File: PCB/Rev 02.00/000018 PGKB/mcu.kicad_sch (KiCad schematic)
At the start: 30 parts, among them U5 RP2040, Y1 12 MHz

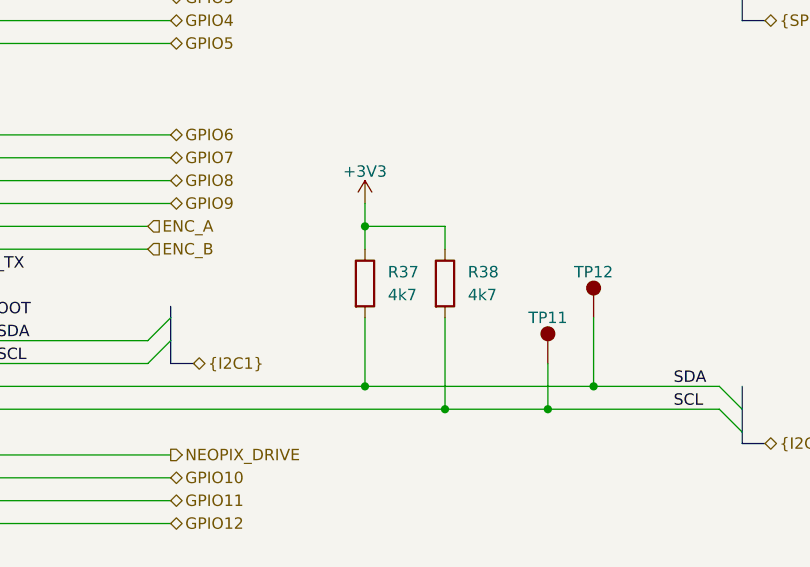
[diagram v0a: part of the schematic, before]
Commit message: step
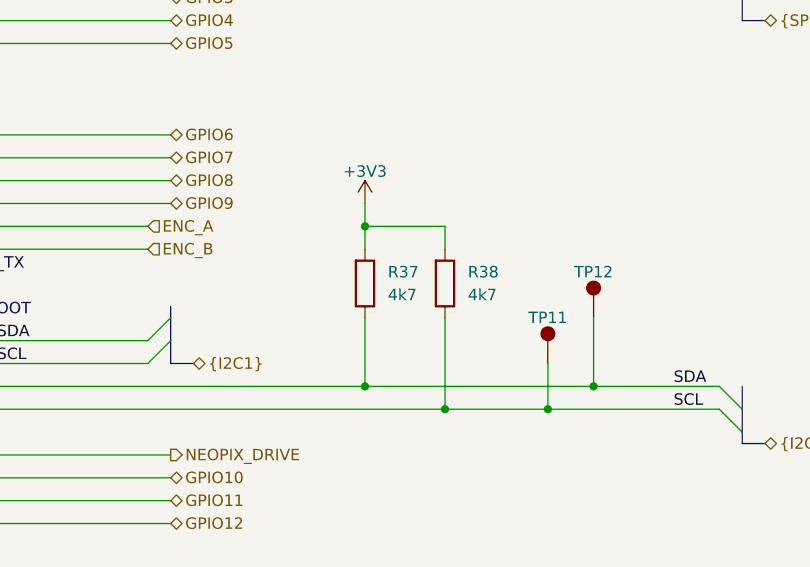
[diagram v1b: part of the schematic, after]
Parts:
- R37, R38: value R_0805_4700_5% -> 4k7; footprint KD_Resistor:RESC2012X50N -> KD_Resistor:RESC1005X40N; symbol KD_Resistor:R_0805_4700_5% -> KD_Resistor:R_0402_4700_1%; MFG_PartNo RMCF0805JT4K70 -> CR0402-FX-4701GLF; Manufacturer Stackpole Electronics Inc -> Bourns Inc.; Supplier_PartNo RMCF0805JT4K70CT-ND -> CR0402-FX-4701GLFCT-ND
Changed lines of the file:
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@@
     (comment 3 "PCB_PN")
   )
+  (bus_alias "QSPI" (members "DATA0" "DATA1" "DATA2" "DATA3" "~{CS}_MEMORY" "CLK"))
   (bus_alias "I2C0" (members "SDA" "SCL"))
   (bus_alias "SPI" (members "SPI_CLK" "SPI_MISO" "SPI_MOSI" "SPI_CS0"))
-  (bus_alias "QSPI" (members "DATA0" "DATA1" "DATA2" "DATA3" "~{CS}_MEMORY" "CLK"))
   (bus_alias "I2C1" (members "I2C1_SDA" "I2C1_SCL"))
   (junction (at 142.24 57.15) (diameter 0) (color 0 0 0 0)
@@
     )
   )
-  (symbol (lib_id "KD_Resistor:R_0805_4700_5%") (at 209.55 116.84 0) (unit 1)
+  (symbol (lib_id "KD_Resistor:R_0402_4700_1%") (at 209.55 116.84 0) (unit 1)
     (in_bom yes) (on_board yes) (dnp no) (fields_autoplaced)
     (property "Reference" "R37" (at 212.09 115.57 0)
       (effects (font (size 1.27 1.27)) (justify left))
     )
-    (property "Value" "R_0805_4700_5%" (at 196.85 85.09 0)
-      (effects (font (size 1.27 1.27)) (justify left) hide)
-    )
-    (property "Footprint" "KD_Resistor:RESC2012X50N" (at 196.85 102.87 0)
-      (effects (font (size 1.27 1.27)) (justify left) hide)
-    )
-    (property "Datasheet" "https://www.seielect.com/catalog/sei-rmcf_rmcp.pdf" (at 196.85 105.41 0)
+    (property "Value" "4k7" (at 196.85 85.09 0)
+      (effects (font (size 1.27 1.27)) (justify left) hide)
+    )
+    (property "Footprint" "KD_Resistor:RESC1005X40N" (at 196.85 102.87 0)
+      (effects (font (size 1.27 1.27)) (justify left) hide)
+    )
+    (property "Datasheet" "https://www.te.com/commerce/DocumentDelivery/DDEController?Action=srchrtrv&DocNm=1773204-3&DocType=DS&DocLang=English" (at 196.85 105.41 0)
       (effects (font (size 1.27 1.27)) (justify left) hide)
     )
@@
       (effects (font (size 1.27 1.27)) (justify left))
     )
-    (property "Manufacturer" "Stackpole Electronics Inc" (at 196.85 87.63 0)
-      (effects (font (size 1.27 1.27)) (justify left) hide)
-    )
-    (property "MFG_PartNo" "RMCF0805JT4K70" (at 196.85 90.17 0)
+    (property "Manufacturer" "Bourns Inc." (at 196.85 87.63 0)
+      (effects (font (size 1.27 1.27)) (justify left) hide)
+    )
+    (property "MFG_PartNo" "CR0402-FX-4701GLF" (at 196.85 90.17 0)
       (effects (font (size 1.27 1.27)) (justify left) hide)
     )
@@
       (effects (font (size 1.27 1.27)) (justify left) hide)
     )
-    (property "Supplier_PartNo" "RMCF0805JT4K70CT-ND" (at 196.85 95.25 0)
+    (property "Supplier_PartNo" "CR0402-FX-4701GLFCT-ND" (at 196.85 95.25 0)
       (effects (font (size 1.27 1.27)) (justify left) hide)
     )
@@
     )
   )
-  (symbol (lib_id "KD_Resistor:R_0805_4700_5%") (at 218.44 116.84 0) (unit 1)
+  (symbol (lib_id "KD_Resistor:R_0402_4700_1%") (at 218.44 116.84 0) (unit 1)
     (in_bom yes) (on_board yes) (dnp no) (fields_autoplaced)
     (property "Reference" "R38" (at 220.98 115.57 0)
       (effects (font (size 1.27 1.27)) (justify left))
     )
-    (property "Value" "R_0805_4700_5%" (at 205.74 85.09 0)
-      (effects (font (size 1.27 1.27)) (justify left) hide)
-    )
-    (property "Footprint" "KD_Resistor:RESC2012X50N" (at 205.74 102.87 0)
-      (effects (font (size 1.27 1.27)) (justify left) hide)
-    )
-    (property "Datasheet" "https://www.seielect.com/catalog/sei-rmcf_rmcp.pdf" (at 205.74 105.41 0)
+    (property "Value" "4k7" (at 205.74 85.09 0)
+      (effects (font (size 1.27 1.27)) (justify left) hide)
+    )
+    (property "Footprint" "KD_Resistor:RESC1005X40N" (at 205.74 102.87 0)
+      (effects (font (size 1.27 1.27)) (justify left) hide)
+    )
+    (property "Datasheet" "https://www.te.com/commerce/DocumentDelivery/DDEController?Action=srchrtrv&DocNm=1773204-3&DocType=DS&DocLang=English" (at 205.74 105.41 0)
       (effects (font (size 1.27 1.27)) (justify left) hide)
     )
@@
       (effects (font (size 1.27 1.27)) (justify left))
     )
-    (property "Manufacturer" "Stackpole Electronics Inc" (at 205.74 87.63 0)
-      (effects (font (size 1.27 1.27)) (justify left) hide)
-    )
-    (property "MFG_PartNo" "RMCF0805JT4K70" (at 205.74 90.17 0)
+    (property "Manufacturer" "Bourns Inc." (at 205.74 87.63 0)
+      (effects (font (size 1.27 1.27)) (justify left) hide)
+    )
+    (property "MFG_PartNo" "CR0402-FX-4701GLF" (at 205.74 90.17 0)
       (effects (font (size 1.27 1.27)) (justify left) hide)
     )
@@
       (effects (font (size 1.27 1.27)) (justify left) hide)
     )
-    (property "Supplier_PartNo" "RMCF0805JT4K70CT-ND" (at 205.74 95.25 0)
-      (effects (font (size 1.27 1.27)) (justify left) hide)
-    )
+    (property "Supplier_PartNo" "CR0402-FX-4701GLFCT-ND" (at 205.74 95.25 0)
+      (effects (font (size 1.27 1.27)) (justify left) hide)
+    )
